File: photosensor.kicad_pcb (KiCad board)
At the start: 2 copper layers, 61 x 45.7 mm, 3 parts, among them P1 TSL1406R, T1 6PIN

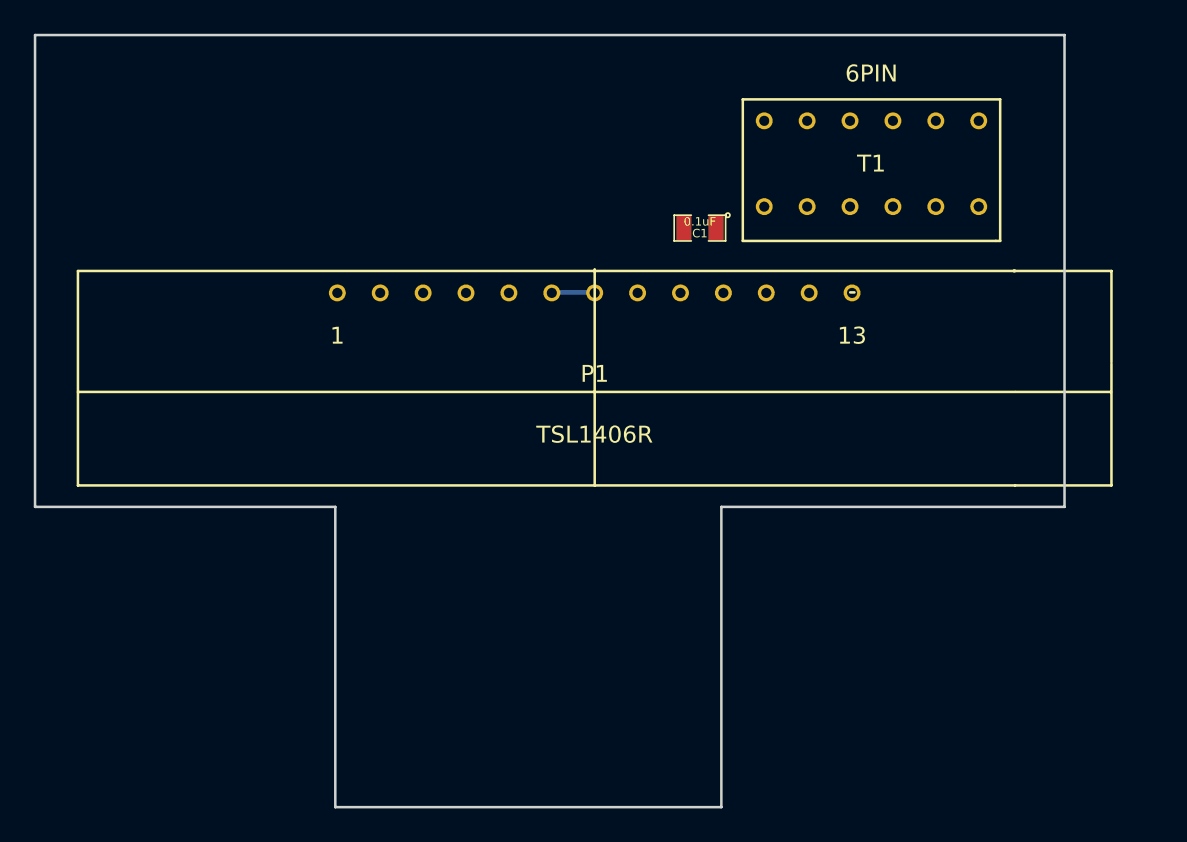
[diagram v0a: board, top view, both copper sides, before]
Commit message: layout
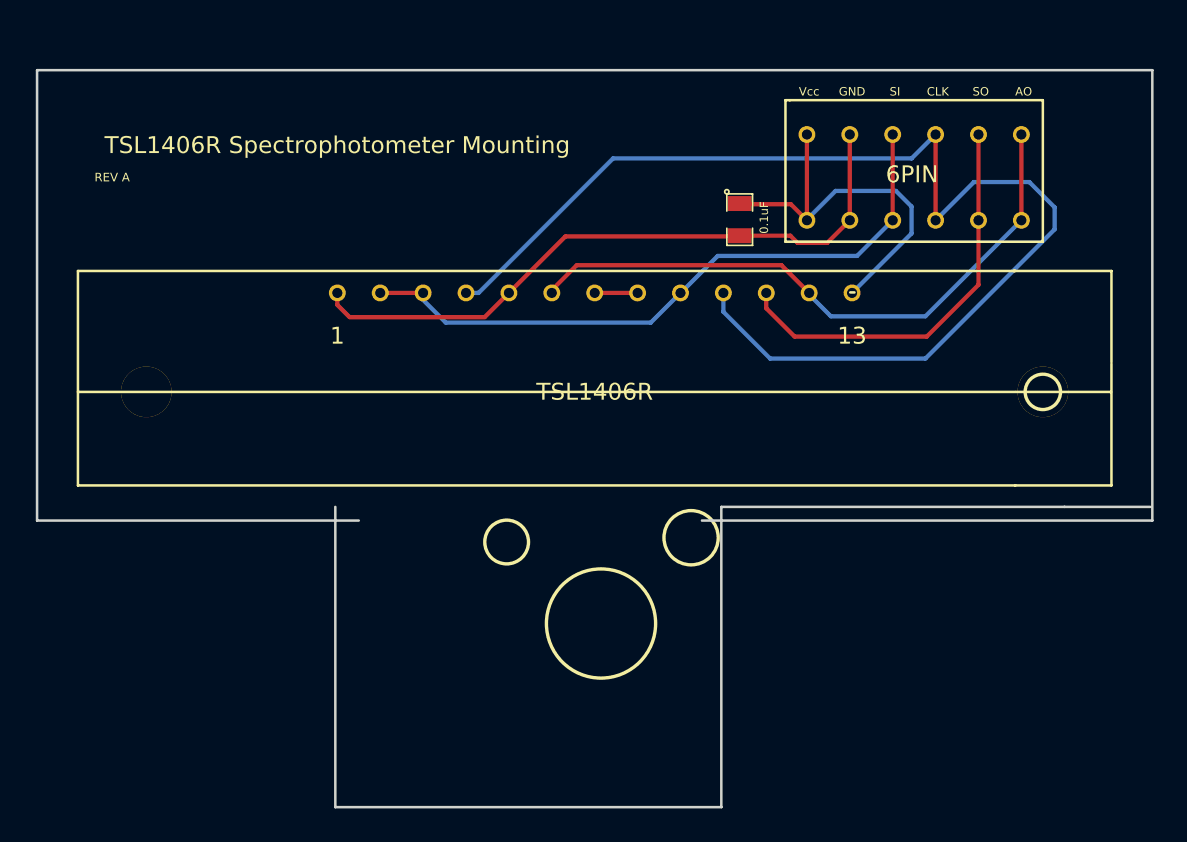
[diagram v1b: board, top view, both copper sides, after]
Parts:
- added ?: , 3mm_drill_hole, F.Cu at (189.5, 121.2)
- added ?: , 3mm_drill_hole, F.Cu at (242.6, 122.7)
- moved ? 6.41 mm to (234.9, 112.6), turned to 0 degrees
- moved ? 2.41 mm to (224.6, 112.5), turned to 270 degrees
- renumbered T1 to ?, C1 to ?, P1 to ?
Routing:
- net N-000003: track 0.00 -> 71.7 mm
- net GND: track 0.00 -> 39.3 mm
- net N-000005: track 0.00 -> 38.9 mm
- net N-000002: track 2.54 -> 37.3 mm
- net N-000001: track 0.00 -> 24.3 mm
- net +5V: track 0.00 -> 23.2 mm
- net N-000004: track 0.00 -> 2.54 mm
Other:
- board size 61 x 45.7 mm -> 66 x 43.6 mm
- board text added: "AO"
- board text added: "CLK"
- board text added: "GND"
- board text added: "REV A"
- board text added: "SI"
- board text added: "SO"
- board text added: "TSL1406R Spectrophotometer Mounting"
- board text added: "Vcc"
